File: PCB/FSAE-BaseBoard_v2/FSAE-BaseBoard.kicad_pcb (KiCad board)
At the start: 2 copper layers, 100 x 100 mm, 71 parts, among them J1 Conn_01x14_Socket, J10 Conn_01x03, J11 Zocalo_Resolver, J12 Bornera_Resolver, J13 Zocalo_Resolver, J14 Screw_Terminal_01x03, J15 Bornera_Encoder, J3 Conn_01x03, J4 Conn_01x02, J5 Conn_01x02, J6 Conn_01x02, J7 Conn_01x02, J8 Conn_01x02, J9 Conn_01x02, K1 Relay_SPDT, Q1 BC817, SW1 SW_Push, SW2 SW_Push, SW3 SW_Push, SW4 SW_Push, U1 ESP32 C3, U10 PC817, U2 ESP32 S3, U3 ISO1050DUB, U4 LM2596S-ADJ, U5 AMS1117-3.3, U6 LoRa SX1278, U7 MPU 6050, U8 PC817, U9 PC817

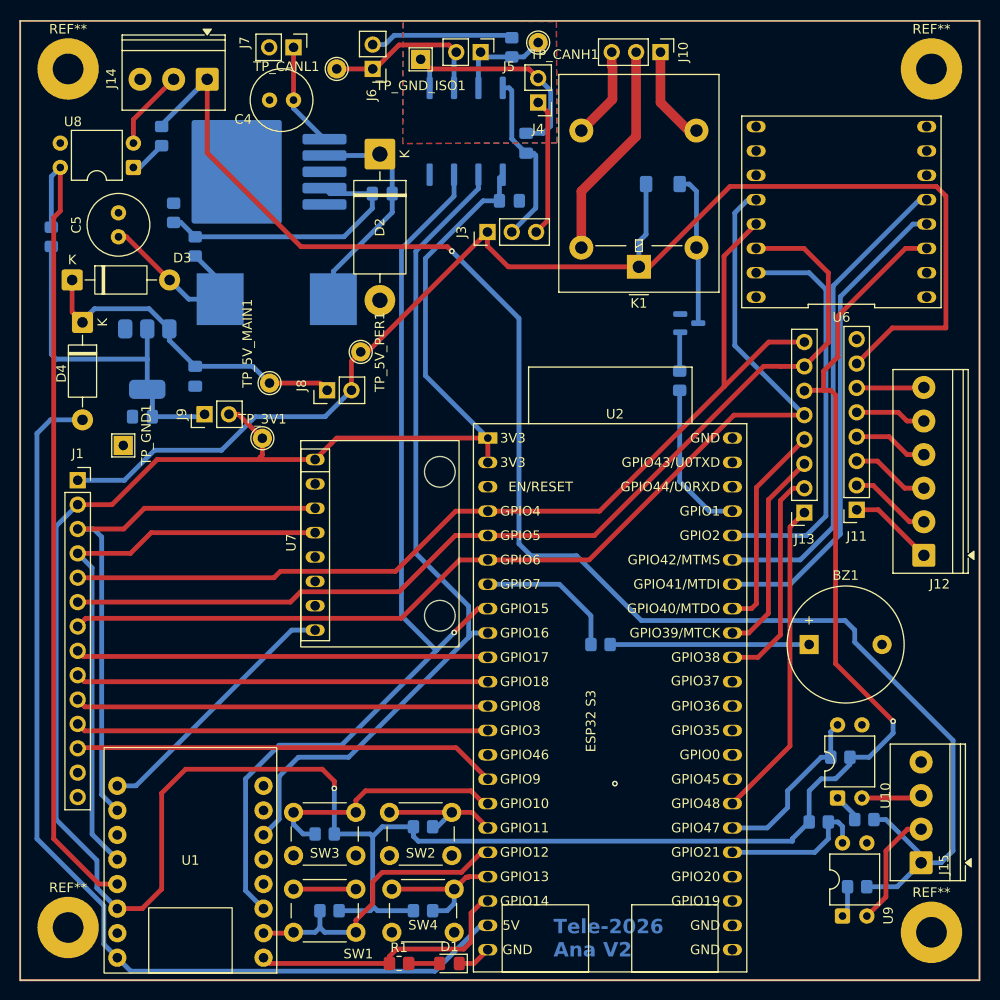
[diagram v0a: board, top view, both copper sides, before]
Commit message: Actualizacion BaseBoard v2
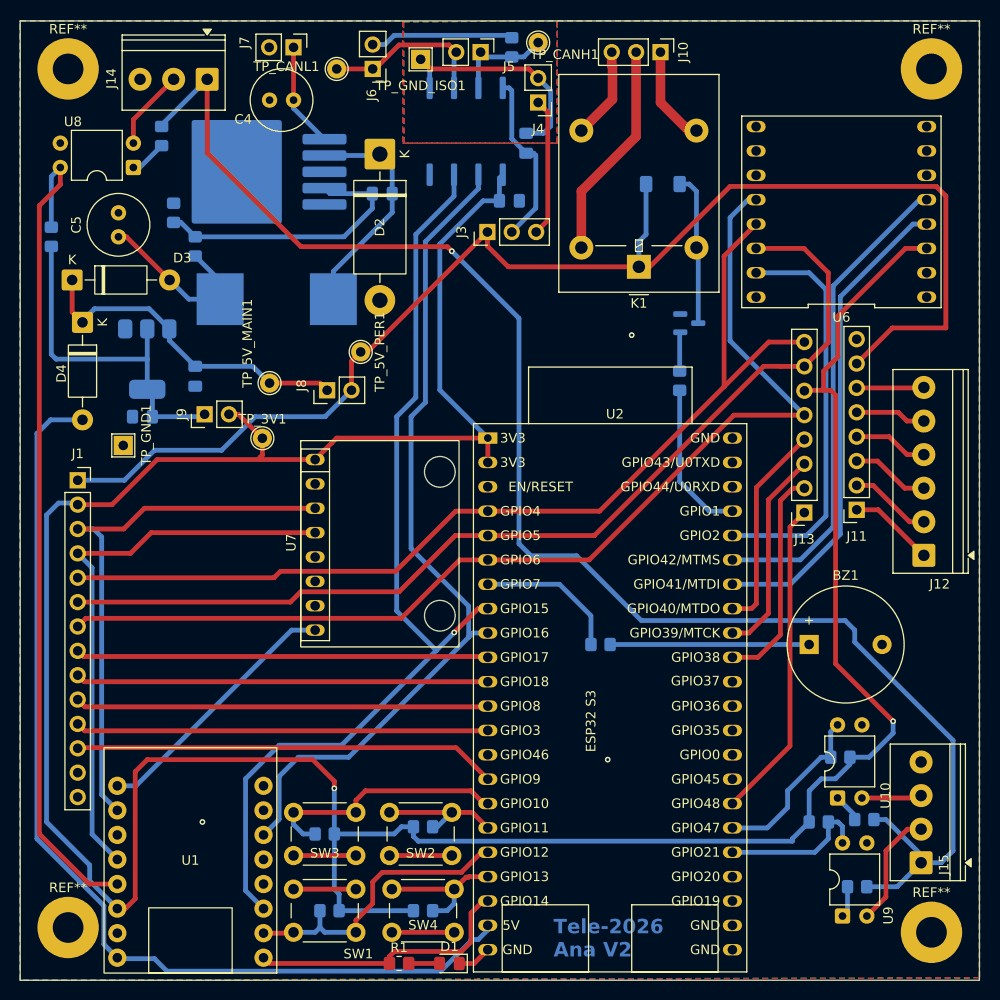
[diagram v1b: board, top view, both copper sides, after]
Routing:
- net GND: track 10.1 -> 29.6 mm, vias 1 -> 3
- net +3.3V: track 356.6 -> 360.4 mm
- net /ESP32 C3 y S3/SENSOR_RPM: track 85.5 -> 87.3 mm
